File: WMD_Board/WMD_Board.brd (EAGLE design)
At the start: 75.8 x 43.7 mm, 71 parts, among them IC1 FGPMMOPA6H, J1 EMPCB.SMAFSTJ.B.HT, Q1 SI2323DS-T1-E3, Q2 SI2323DS-T1-E3, Q3 SI2312BDS, U1 STM32L053C8T6, U2 BSS138, U3 RFM69HCW, U4 BSS138, U6 TPS72218DBVR, U7 M24512-DRMN8TP/K, Y2 ABS06-107-32.768KHZ-T

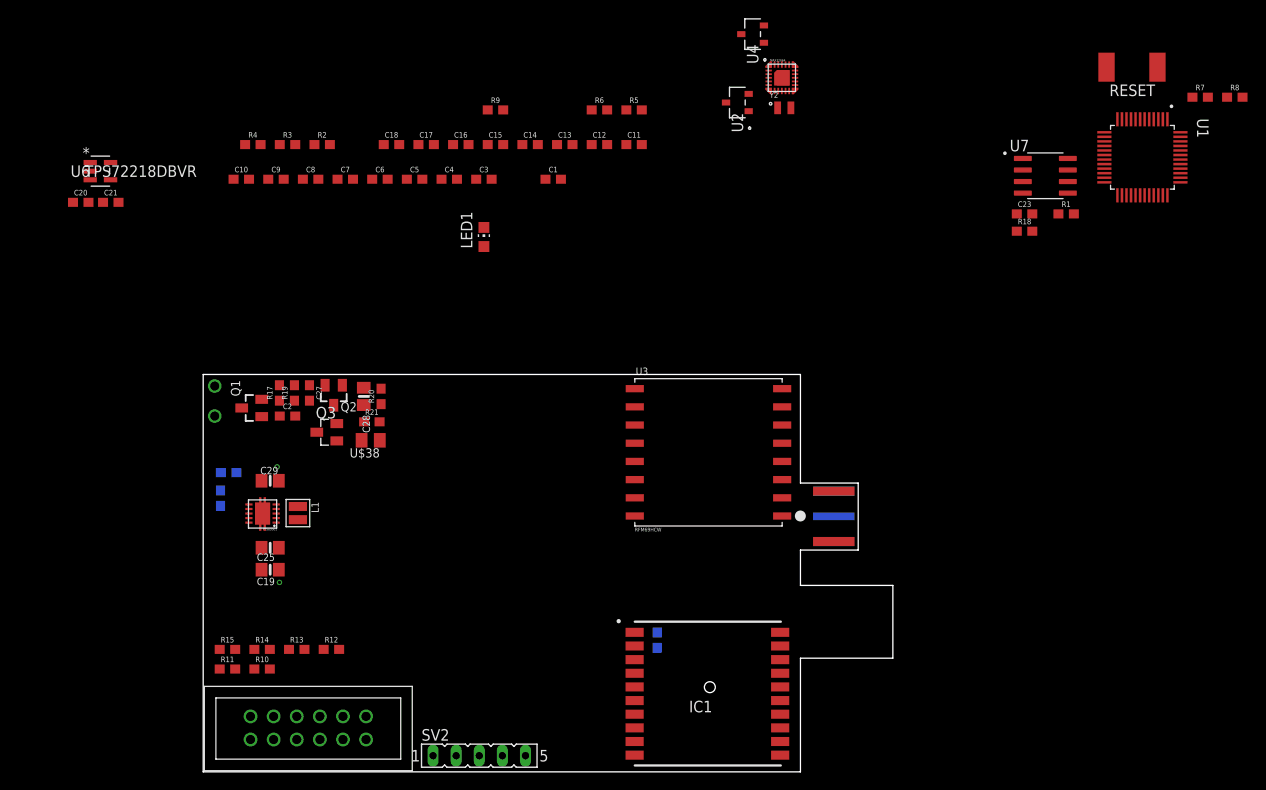
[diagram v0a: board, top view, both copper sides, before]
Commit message: lots of routing stuff
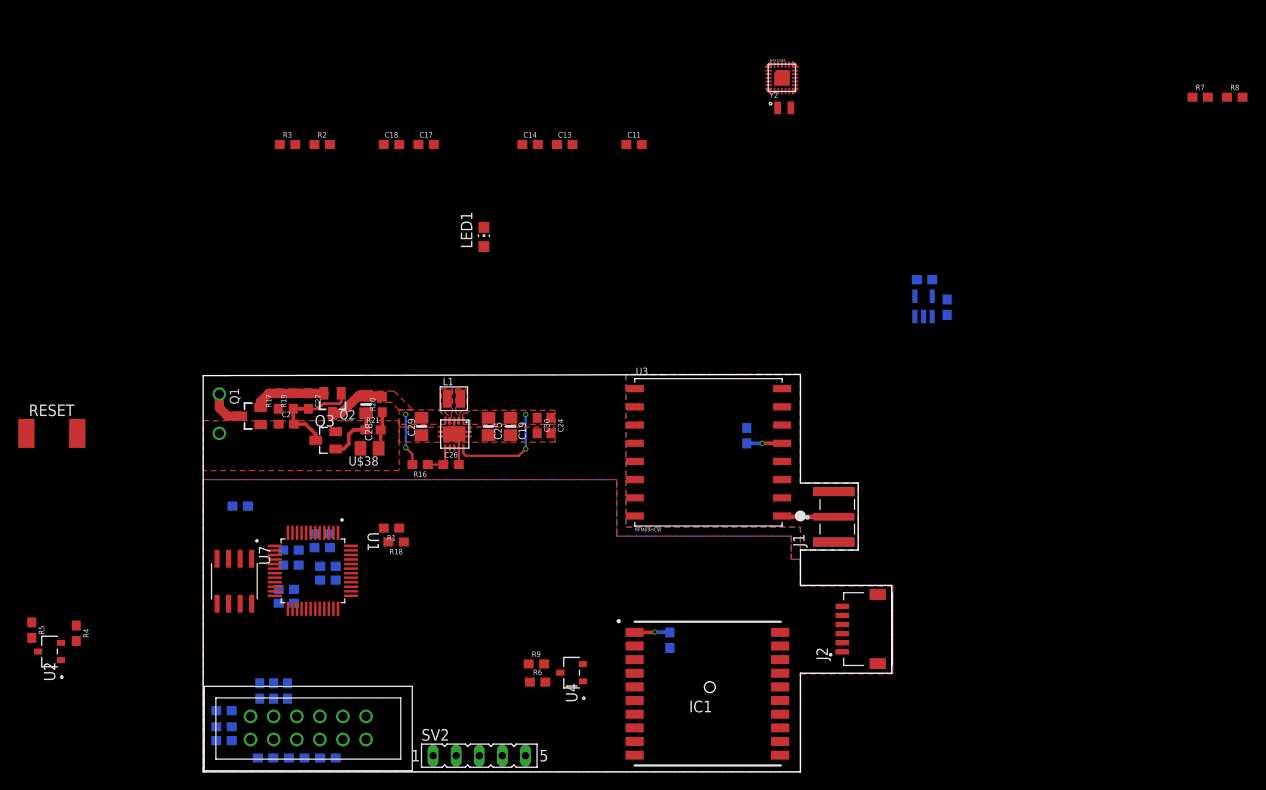
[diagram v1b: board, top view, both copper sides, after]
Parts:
- added C24: 0.01uF, SparkFun-Capacitors:0603
- added C30: 0.1uF, SparkFun-Capacitors:0603
- added J2: 5015680607, WMD_TO_HRF:MOLEX_5015680607
- R4, R5, R6, R9: value 1k -> 4.7k
- moved RESET 125.4 mm to (-16.6, 37.2), turned to 0 degrees
- moved U1 101.9 mm to (12.1, 22.1)
- moved U7 99.7 mm to (3.43, 21.0), turned to 270 degrees
- moved U2 96.7 mm to (-16.9, 13.2)
- moved C20 93.2 mm to (79.3, 54.1), flipped to the bottom
- moved C21 92.7 mm to (81.8, 51.1), flipped to the bottom, turned to 90 degrees
- moved C23 92.0 mm to (4.06, 29.2), flipped to the bottom
- moved U6 91.7 mm to (79.2, 51.2), flipped to the bottom, turned to 90 degrees
- moved R5 87.5 mm to (-18.8, 15.6), turned to 270 degrees
- moved R1 81.8 mm to (20.7, 26.8), turned to 180 degrees
- moved R18 77.1 mm to (21.2, 25.3), turned to 180 degrees
- moved U4 73.0 mm to (40.5, 10.9)
- moved C5 64.3 mm to (13.7, 1.52), flipped to the bottom, turned to 180 degrees
- moved C4 63.5 mm to (2.29, 6.73), flipped to the bottom
- moved R6 63.3 mm to (36.8, 9.87)
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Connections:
- removed net BTN_2_2: C3.2
- removed net BTN_3_2: C4.2
- removed net BTN_4_2: C5.2
- net 1.8V: now also J2.1
- net 3.3V: now also C24.1, C30.1, J2.3
- net GND: now also C24.2, C3.2, C30.2, C4.2, C5.2, J2.6
- net INT: now also J2.2
- net SCL_TO_HR_SENSOR: now also J2.5
- net SDA_TO_HR_SENSOR: now also J2.4
- net WC_EEPROM: now also U1.20; no longer U1.46
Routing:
- net 3.3V: track 0.00 -> 19.6 mm, vias 0 -> 4
- net VIN_BB: track 0.00 -> 12.2 mm, vias 0 -> 2
- net N$14: track 0.00 -> 11.8 mm
- net MEASURE: track 0.00 -> 7.99 mm
- net N$13: track 0.00 -> 6.60 mm
- net N$8: track 0.00 -> 5.71 mm
- net GND: track 0.00 -> 5.06 mm
- net N$7: track 0.00 -> 4.76 mm
- net VIN_BATTERY: track 0.00 -> 4.22 mm
- net SHUTDOWN: track 0.00 -> 4.14 mm
- added copper zone on layer 1, net 3.3V
- added copper zone on layer 1, net GND
- added copper zone on layer 16, net GND
- added copper zone on layer 1, net N$2
- added copper zone on layer 1, net N$3
- added copper zone on layer 1, net VIN_BB
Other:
- board size 75.8 x 43.7 mm -> 75.7 x 43.7 mm
